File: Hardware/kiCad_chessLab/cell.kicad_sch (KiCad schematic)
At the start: 4 parts, among them IC5 SS49E

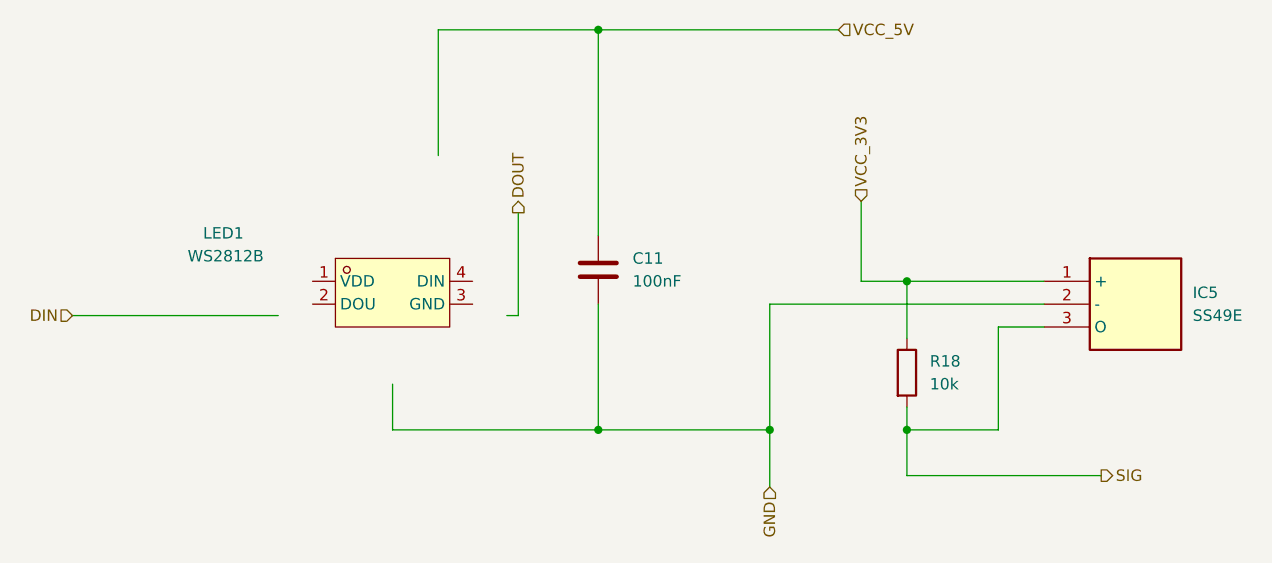
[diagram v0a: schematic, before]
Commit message: Usb c new design
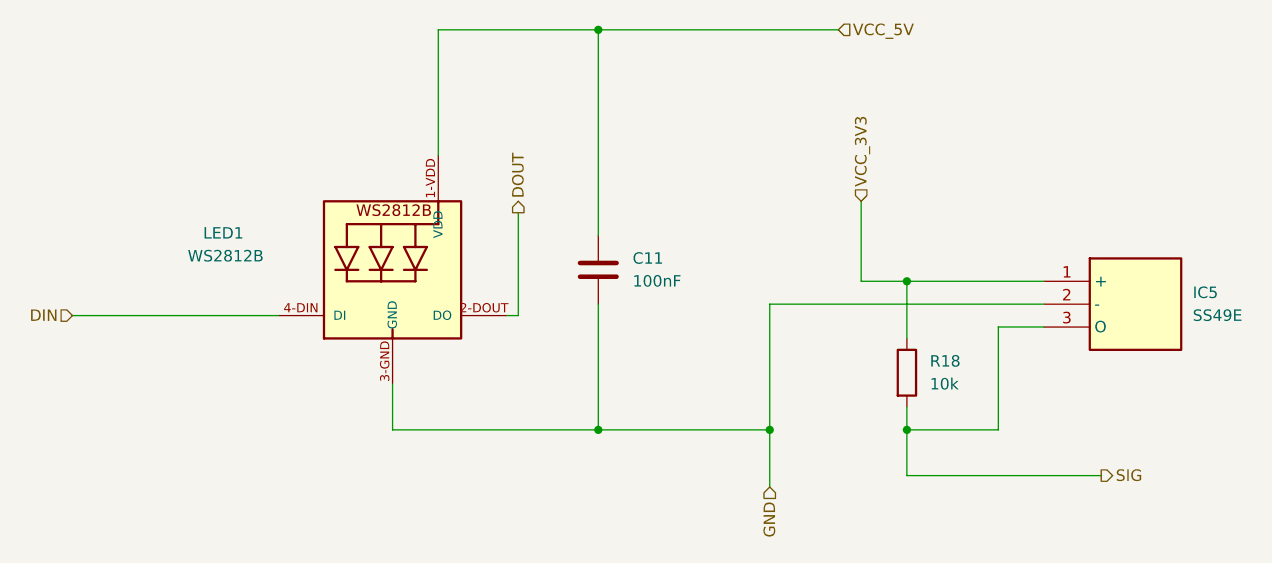
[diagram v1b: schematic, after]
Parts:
- LED1: footprint chessLab-footprints:LED-SMD_4P-L5.0-W5.0-BL_XL-5050RGBC -> chessLab-footprints:WS2812B; symbol chessLab-symbols:XL-5050RGBC-WS2812B -> chessLab-symbols:WS2812B
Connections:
- net DIN: now also LED1.4-DIN (DI)
- net DOUT: now also LED1.2-DOUT (DO)
- net GND: now also LED1.3-GND (GND)
- net VCC_5V: now also LED1.1-VDD (VDD)
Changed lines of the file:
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@@
 	)
 	(symbol
-		(lib_id "chessLab-symbols:XL-5050RGBC-WS2812B")
+		(lib_id "chessLab-symbols:WS2812B")
 		(at 64.77 66.04 0)
 		(unit 1)
@@
 			)
 		)
-		(property "Footprint" "chessLab-footprints:LED-SMD_4P-L5.0-W5.0-BL_XL-5050RGBC"
+		(property "Footprint" "chessLab-footprints:WS2812B"
 			(at 64.77 66.04 0)
 			(hide yes)
